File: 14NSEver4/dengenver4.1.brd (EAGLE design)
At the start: 80 x 25.4 mm, 44 parts, among them Q1 16mhz, SW2 SRIDE_SWITCH

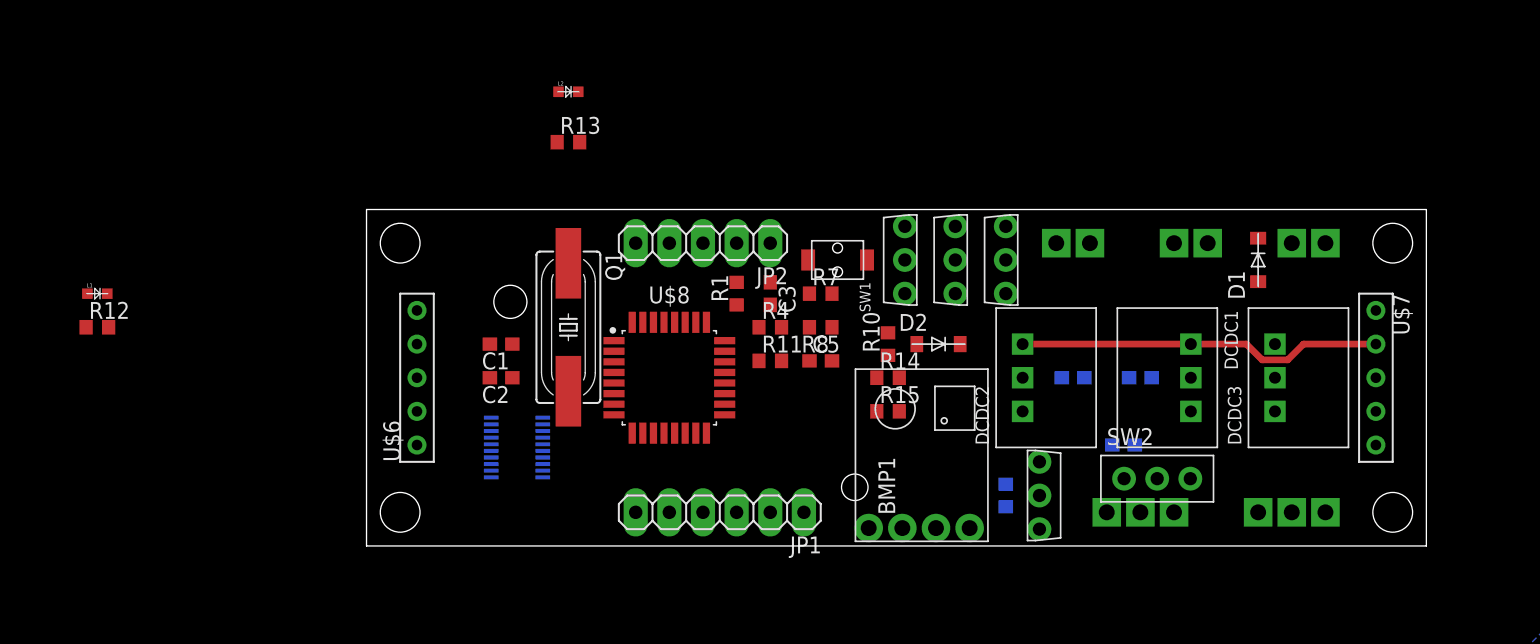
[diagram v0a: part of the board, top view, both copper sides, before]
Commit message: changed board files
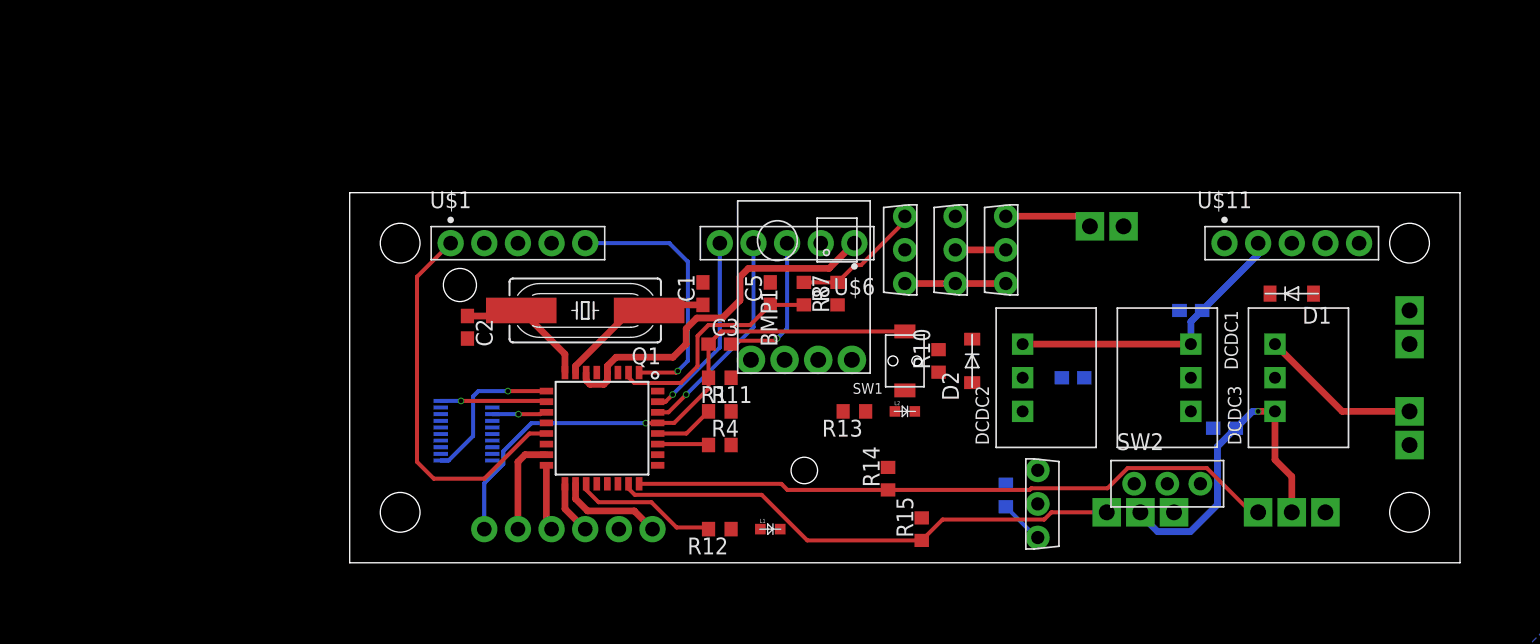
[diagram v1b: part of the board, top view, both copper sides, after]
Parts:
- removed JP1: (no value), pinhead:1X06
- removed JP2: (no value), pinhead:1X05
- removed U$8: ATMEGA328P-AU, ATMEGA328P-AU:QFP80P900X900X120-32N
- added U$1, U$11: 1X5, pin_socket:HDRVR5W64P254_1X5_1310X250X865B
- added U$10: 1X61X6_2.5, pin_socket:HDRVR6W64P254_1X6_1564X250X865B
- U$6: device PinSocket:1X5 -> pin_socket:HDRVR5W64P254_1X5_1310X250X865B
- U$7: value 1X5 -> ATMEGA328P-AUATMEGA328P-AU; device PinSocket:1X5 -> ATMEGA328P-AU:ATMEGA328P-AU
- moved U$7 59.1 mm to (17.8, 8.89)
- moved L1 53.8 mm to (30.5, 1.27)
- moved R12 49.4 mm to (26.7, 1.27), turned to 180 degrees
- moved U$6 36.4 mm to (36.8, 22.9), turned to 180 degrees
- moved L2 35.0 mm to (40.6, 10.2)
- moved R13 29.6 mm to (36.8, 10.2), turned to 180 degrees
- moved CON5 26.2 mm to (78.7, 16.5), turned to 90 degrees
- moved CON4 15.9 mm to (78.7, 8.89), turned to 90 degrees
- moved C1 15.7 mm to (25.4, 19.1), turned to 90 degrees
- moved BMP1 15.5 mm to (33.0, 19.1)
- moved R4 9.67 mm to (26.7, 7.62)
- moved R15 9.25 mm to (41.9, 1.27), turned to 90 degrees
- moved SW1 9.16 mm to (40.6, 14.0), turned to 180 degrees
- moved C7 7.73 mm to (64.8, 8.89)
- moved R14 7.62 mm to (39.4, 5.08), turned to 90 degrees
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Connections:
- removed net LED1.0: R13.2
- removed net LED1.1: R12.2
- new net LED_1.1: R12.2, U$7.P$19
- net +3V3: now also U$1.2, U$11.1; no longer U$6.P$2, U$7.P$1
- net +5V: now also U$1.3, U$10.1, U$11.2, U$6.1, U$7.P$18, U$7.P$4, U$7.P$6; no longer JP1.1, JP2.1, U$6.P$3, U$7.P$2, U$8.AVCC, U$8.VCC1, U$8.VCC2
- net BORD1: now also U$1.5, U$7.P$1; no longer U$6.P$5, U$8.PD3
- net BORD2: now also U$1.1, U$7.P$13; no longer U$6.P$1, U$8.PB1
- net BORDRX: now also U$11.3, U$7.P$26; no longer U$7.P$3, U$8.PC3
- net BORDTX: now also U$11.4, U$7.P$25; no longer U$7.P$4, U$8.PC2
- net FP_CHECKER: now also U$7.P$2; no longer U$8.PD4
- net GND: now also U$1.4, U$10.2, U$11.5, U$6.2, U$7.P$21, U$7.P$3; no longer JP1.2, JP2.2, U$6.P$4, U$8.GND1, U$8.GND2, U$8.GND3
- net IM_BUSY: now also U$7.P$10; no longer U$8.PD6
- net IM_RESET: now also U$7.P$9; no longer U$8.PD5
- net LED_1.0: now also R13.2, U$7.P$32; no longer U$8.PD2
- net MISO: now also U$10.4, U$7.P$16; no longer JP1.4, U$8.PB4
- net MOSI: now also U$10.5, U$7.P$15; no longer JP1.5, U$8.PB3
- net N$12: now also U$7.P$7; no longer U$8.PB6
- net N$13: now also U$7.P$8; no longer U$8.PB7
- net RESET: now also U$6.3; no longer JP2.3
- net RESETB: now also U$10.6, U$7.P$29; no longer JP1.6, U$8.PC6
- net RX: now also U$6.4, U$7.P$30; no longer JP2.4, U$8.PD0
- net RX_IM: now also U$7.P$11; no longer U$8.PD7
- net SCK: now also U$10.3, U$7.P$17; no longer JP1.3, U$8.PB5
- net SCL: now also U$7.P$28; no longer U$8.PC5
- net SDA: now also U$7.P$27; no longer U$8.PC4
- net SERVO1: now also U$7.P$24; no longer U$8.PC1
- net SERVO2: now also U$7.P$23; no longer U$8.PC0
- net SS: now also U$7.P$14; no longer U$8.PB2
- net TX: now also U$6.5, U$7.P$31; no longer JP2.5, U$8.PD1
- net TX_RM: now also U$7.P$12; no longer U$8.PB0
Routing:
- net SERVO1: track 0.00 -> 49.0 mm
- net RESETB: track 0.00 -> 42.5 mm, vias 0 -> 1
- net SERVO2: track 0.00 -> 39.0 mm
- net +5V: track 27.7 -> 58.1 mm
- net BORD2: track 0.00 -> 29.3 mm
- net SERVO5V: track 0.00 -> 25.3 mm, vias 0 -> 1
- net BORD1: track 0.00 -> 19.9 mm, vias 0 -> 1
- net FP_CHECKER: track 0.00 -> 17.8 mm
- net RX: track 0.00 -> 16.2 mm, vias 0 -> 1
- net TX: track 0.00 -> 14.3 mm, vias 0 -> 1
- net SERVORAW: track 0.00 -> 12.3 mm
- net N$12: track 0.00 -> 12.0 mm
- net IM_RESET: track 0.00 -> 11.9 mm, vias 0 -> 1
- net RESET: track 0.00 -> 11.2 mm, vias 0 -> 1
- net LED_1.1: track 0.00 -> 10.9 mm
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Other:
- board size 80 x 25.4 mm -> 83.8 x 27.9 mm
